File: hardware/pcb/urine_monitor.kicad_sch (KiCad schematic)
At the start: 27 parts, among them J1 LoadCell, J2 EInk_FPC, J3 USB-C_Power, Q1 SI2301, Q2 2N7002, SW1 USER_BTN, U1 RAK3172, U2 HX711, U3 TPS61220, U4 MIC5504-3.3

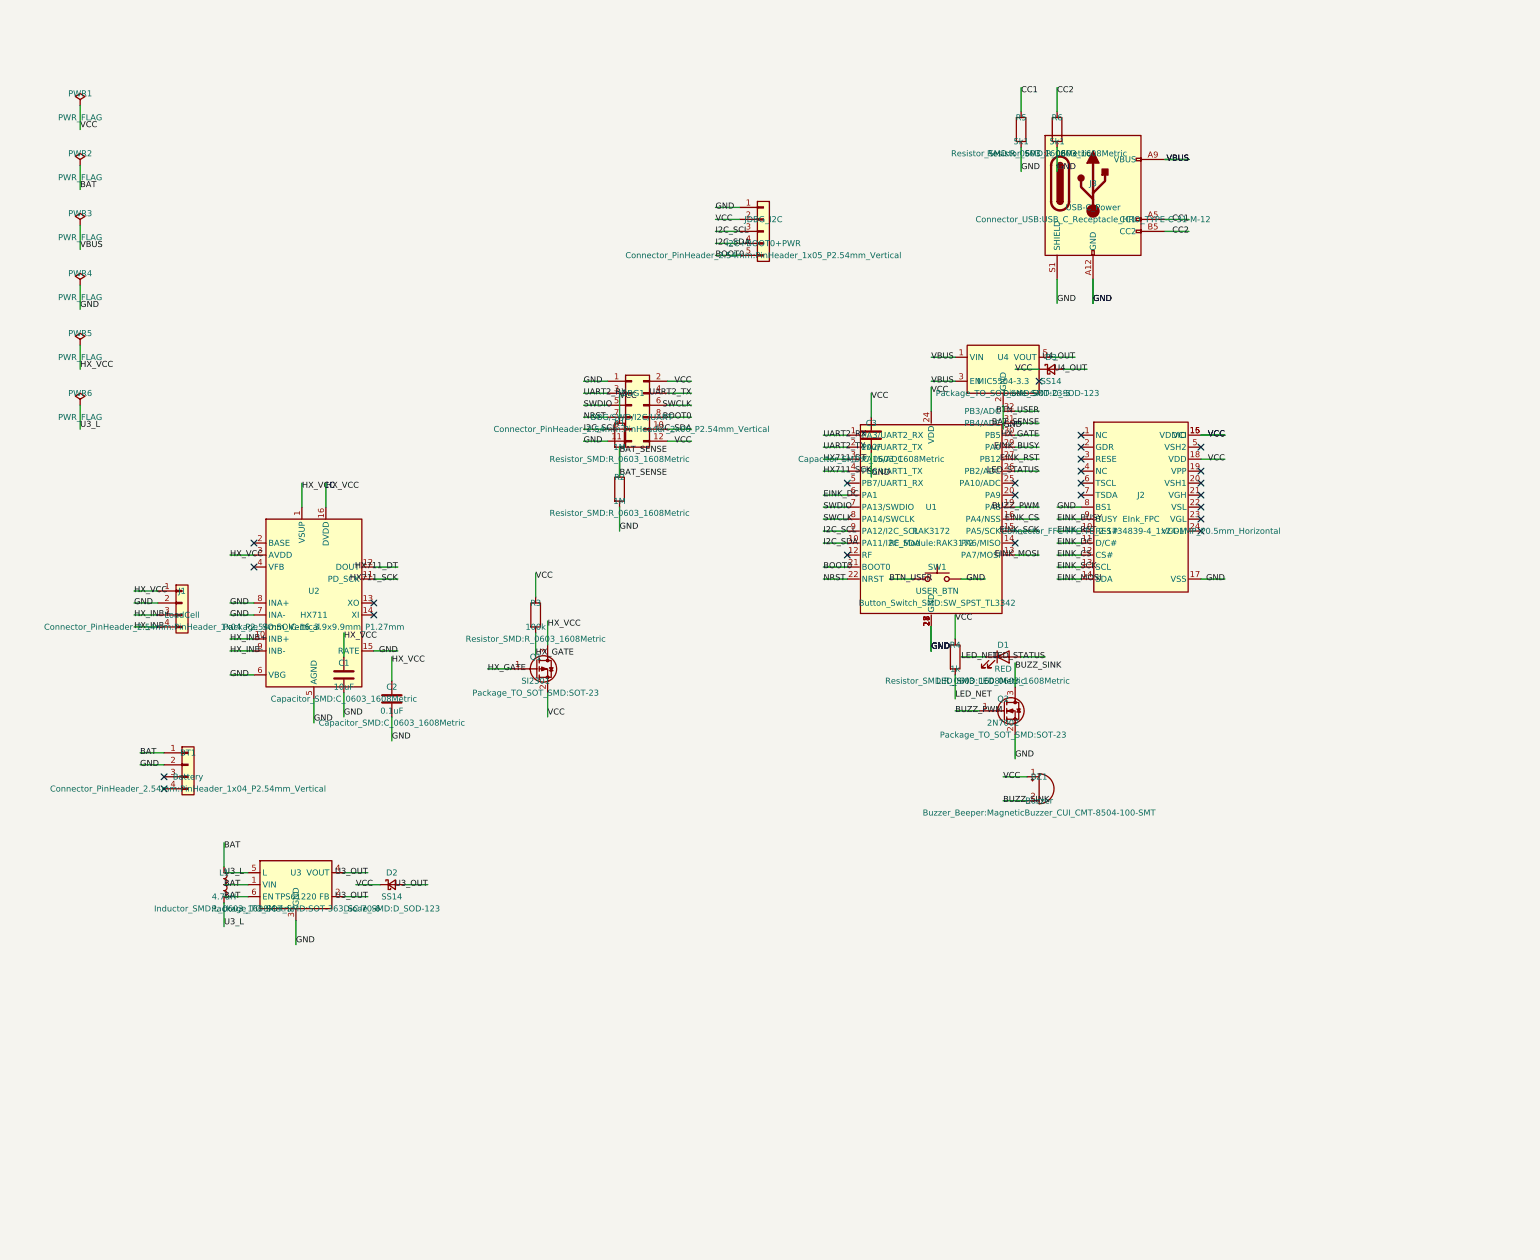
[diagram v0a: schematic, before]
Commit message: init
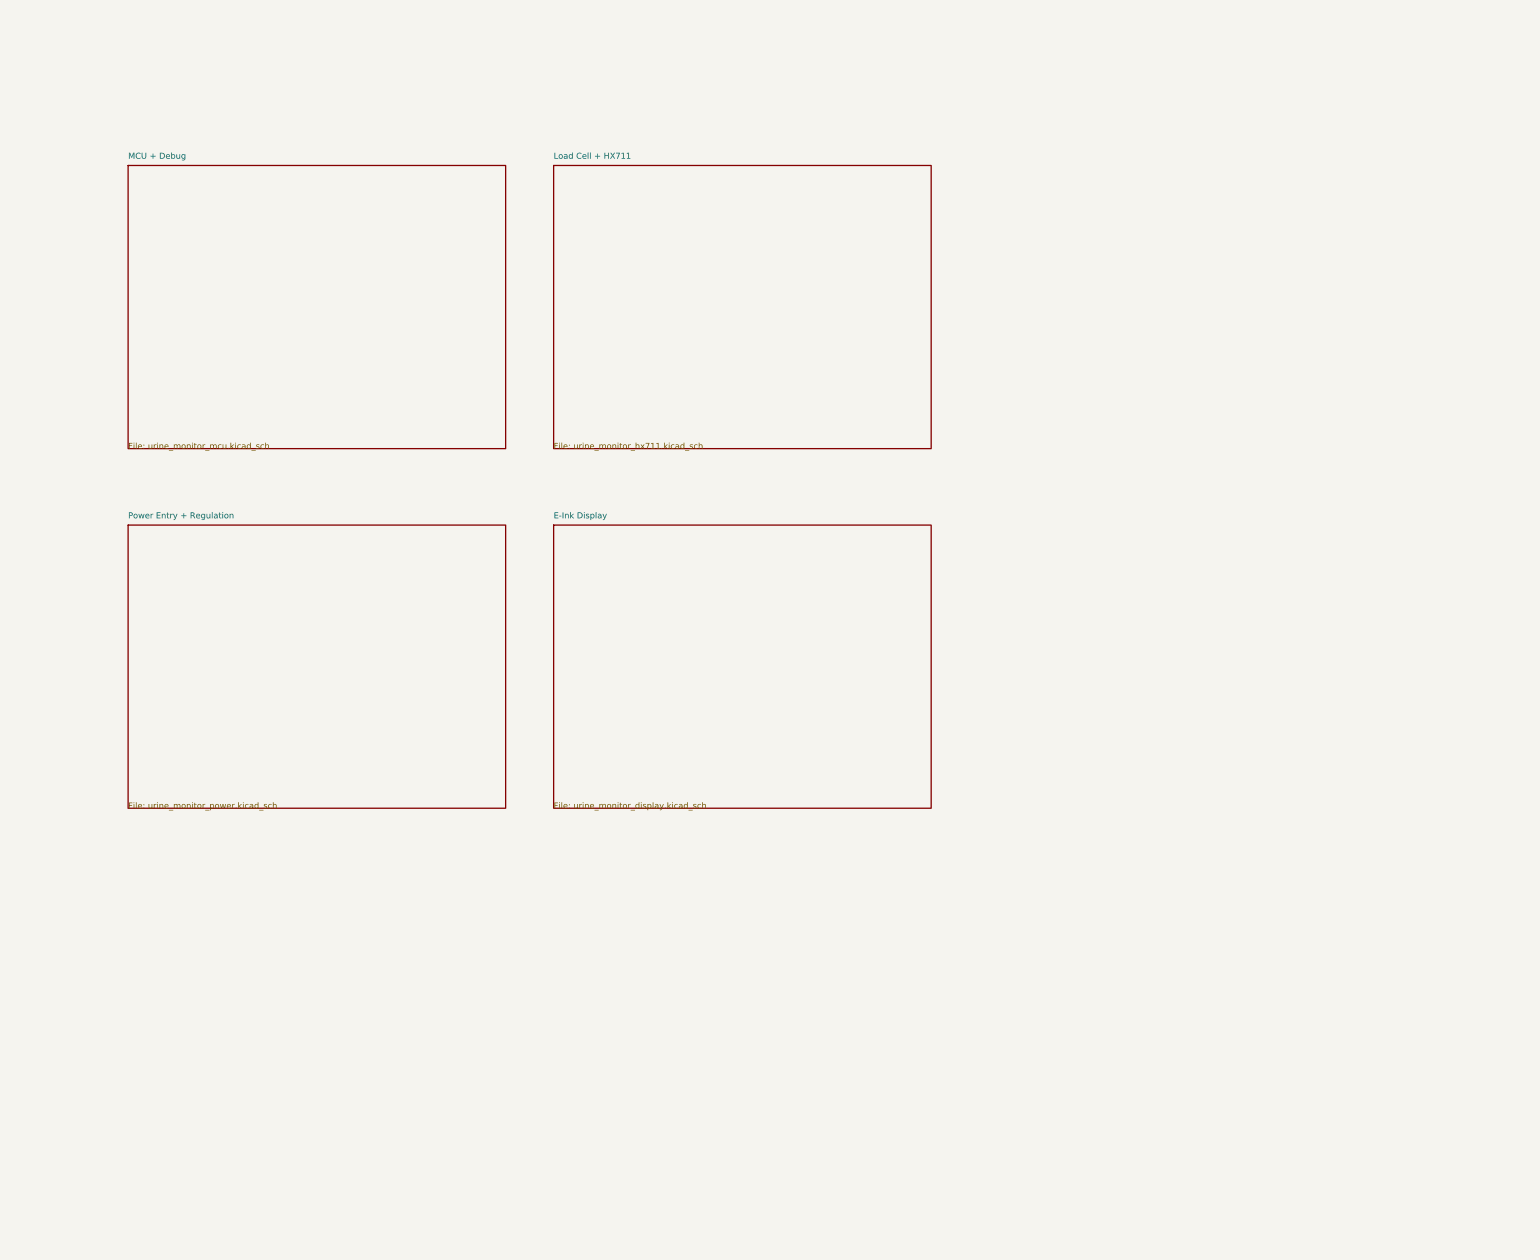
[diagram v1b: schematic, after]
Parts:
- removed BT1: Battery, Connector_PinHeader_2.54mm:PinHeader_1x04_P2.54mm_Vertical, symbol Connector_Generic:Conn_01x04
- removed BZ1: Buzzer, Buzzer_Beeper:MagneticBuzzer_CUI_CMT-8504-100-SMT, symbol Device:Buzzer
- removed C1, C3: 10uF, Capacitor_SMD:C_0603_1608Metric, symbol Device:C
- removed C2: 0.1uF, Capacitor_SMD:C_0603_1608Metric, symbol Device:C
- removed D1: RED, LED_SMD:LED_0603_1608Metric, symbol Device:LED
- removed D2, D3: SS14, Diode_SMD:D_SOD-123, symbol Device:D_Schottky_Small
- removed J1: LoadCell, Connector_PinHeader_2.54mm:PinHeader_1x04_P2.54mm_Vertical, symbol Connector_Generic:Conn_01x04
- removed J2: EInk_FPC, Connector_FFC-FPC:TE_2-1734839-4_1x24-1MP_P0.5mm_Horizontal, symbol Project_Lib:GDEY0213B74
- removed J3: USB-C_Power, Connector_USB:USB_C_Receptacle_HRO_TYPE-C-31-M-12, symbol Connector:USB_C_Receptacle_PowerOnly_6P
- removed JDBG1: DBG/SWD/I2C/UART, Connector_PinHeader_2.54mm:PinHeader_2x06_P2.54mm_Vertical, symbol Connector_Generic:Conn_02x06_Odd_Even
- removed JDBG_I2C: I2C+BOOT0+PWR, Connector_PinHeader_2.54mm:PinHeader_1x05_P2.54mm_Vertical, symbol Connector_Generic:Conn_01x05
- removed L1: 4.7uH, Inductor_SMD:L_0603_1608Metric, symbol Device:L
- removed Q1: SI2301, Package_TO_SOT_SMD:SOT-23, symbol Transistor_FET:Q_PMOS_GSD
- removed Q2: 2N7002, Package_TO_SOT_SMD:SOT-23, symbol Transistor_FET:Q_NMOS_GSD
- removed R1, R2: 1M, Resistor_SMD:R_0603_1608Metric, symbol Device:R
- removed R3: 100k, Resistor_SMD:R_0603_1608Metric, symbol Device:R
- removed R4: 1k, Resistor_SMD:R_0603_1608Metric, symbol Device:R
- removed R5, R6: 5k1, Resistor_SMD:R_0603_1608Metric, symbol Device:R
- removed SW1: USER_BTN, Button_Switch_SMD:SW_SPST_TL3342, symbol Switch:SW_Push
- removed U1: RAK3172, RF_Module:RAK3172, symbol Project_Lib:RAK3172
- removed U2: HX711, Package_SO:SOIC-16_3.9x9.9mm_P1.27mm, symbol Analog_ADC:HX711
- removed U3: TPS61220, Package_TO_SOT_SMD:SOT-363_SC-70-6, symbol Regulator_Switching:TPS61220DCK
- removed U4: MIC5504-3.3, Package_TO_SOT_SMD:SOT-23-5, symbol Regulator_Linear:MIC5504-3.3YM5
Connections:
- no-connect marks 25 -> 0
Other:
- added sheet E-Ink Display (urine_monitor_display.kicad_sch)
- added sheet Load Cell + HX711 (urine_monitor_hx711.kicad_sch)
- added sheet MCU + Debug (urine_monitor_mcu.kicad_sch)
- added sheet Power Entry + Regulation (urine_monitor_power.kicad_sch)
- title: (none) -> Urine Monitor

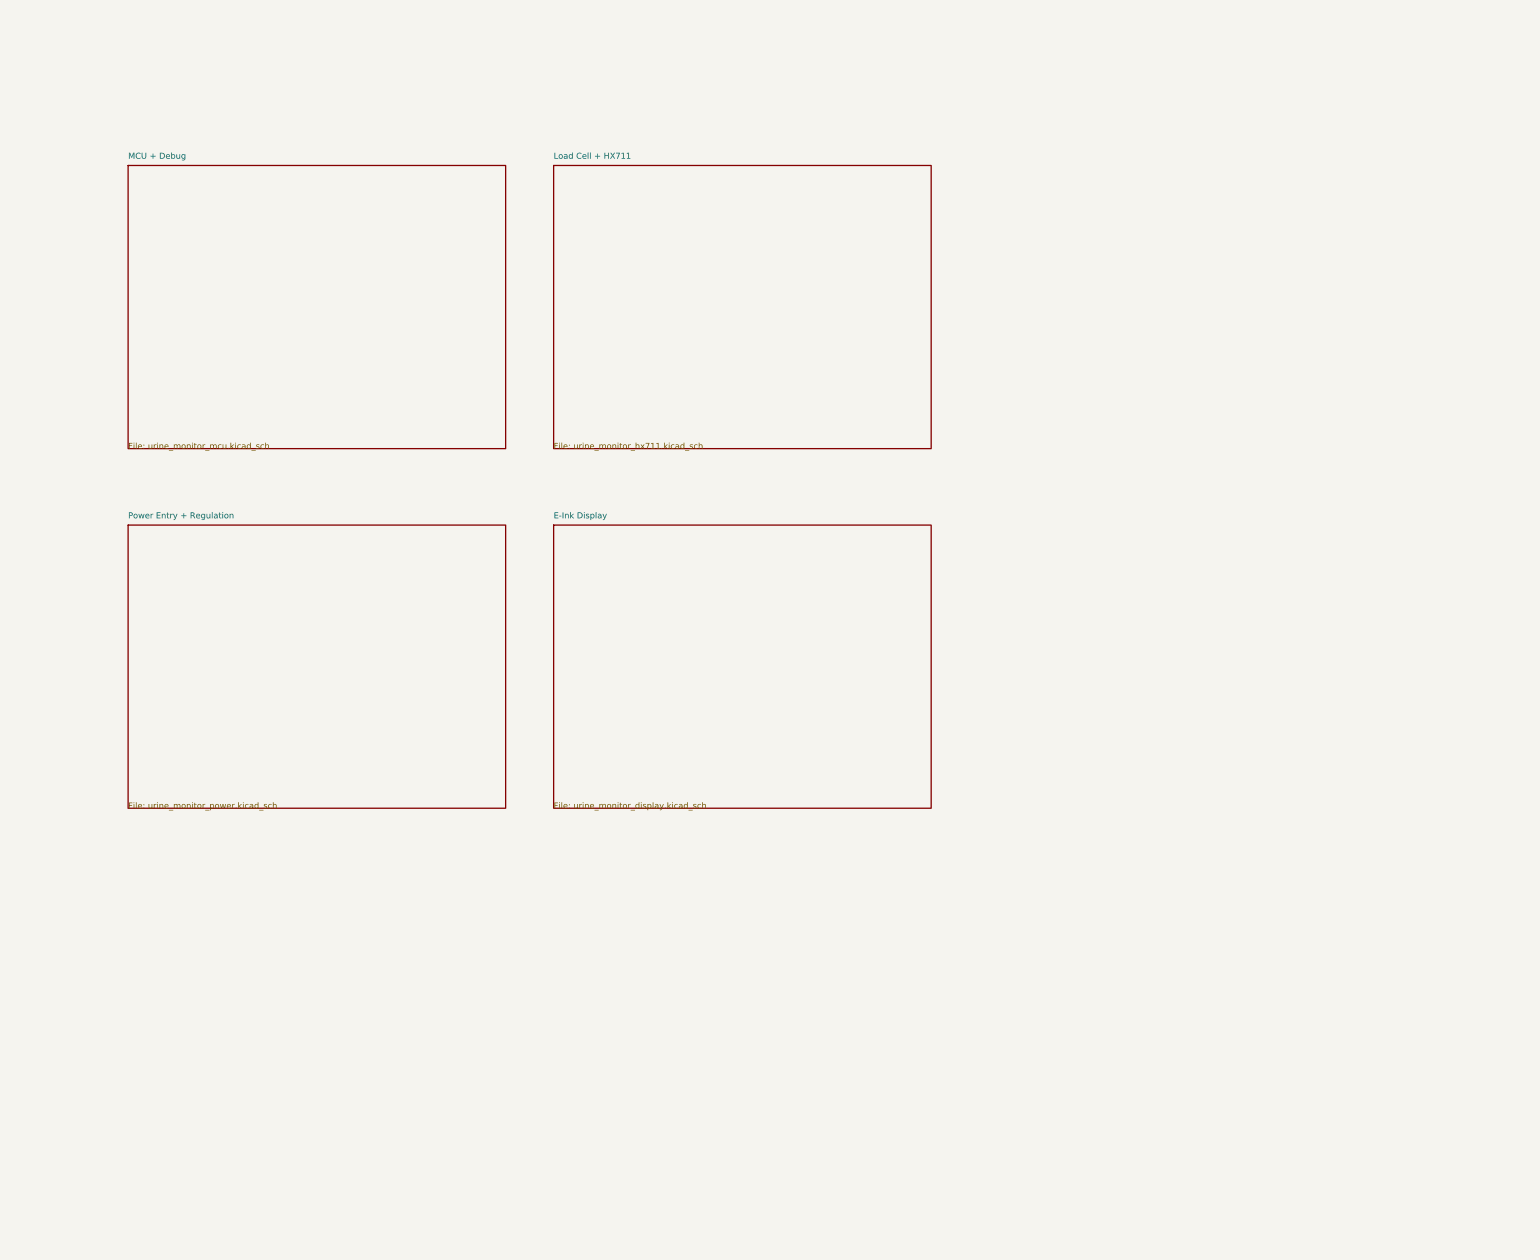
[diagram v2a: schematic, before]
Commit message: init
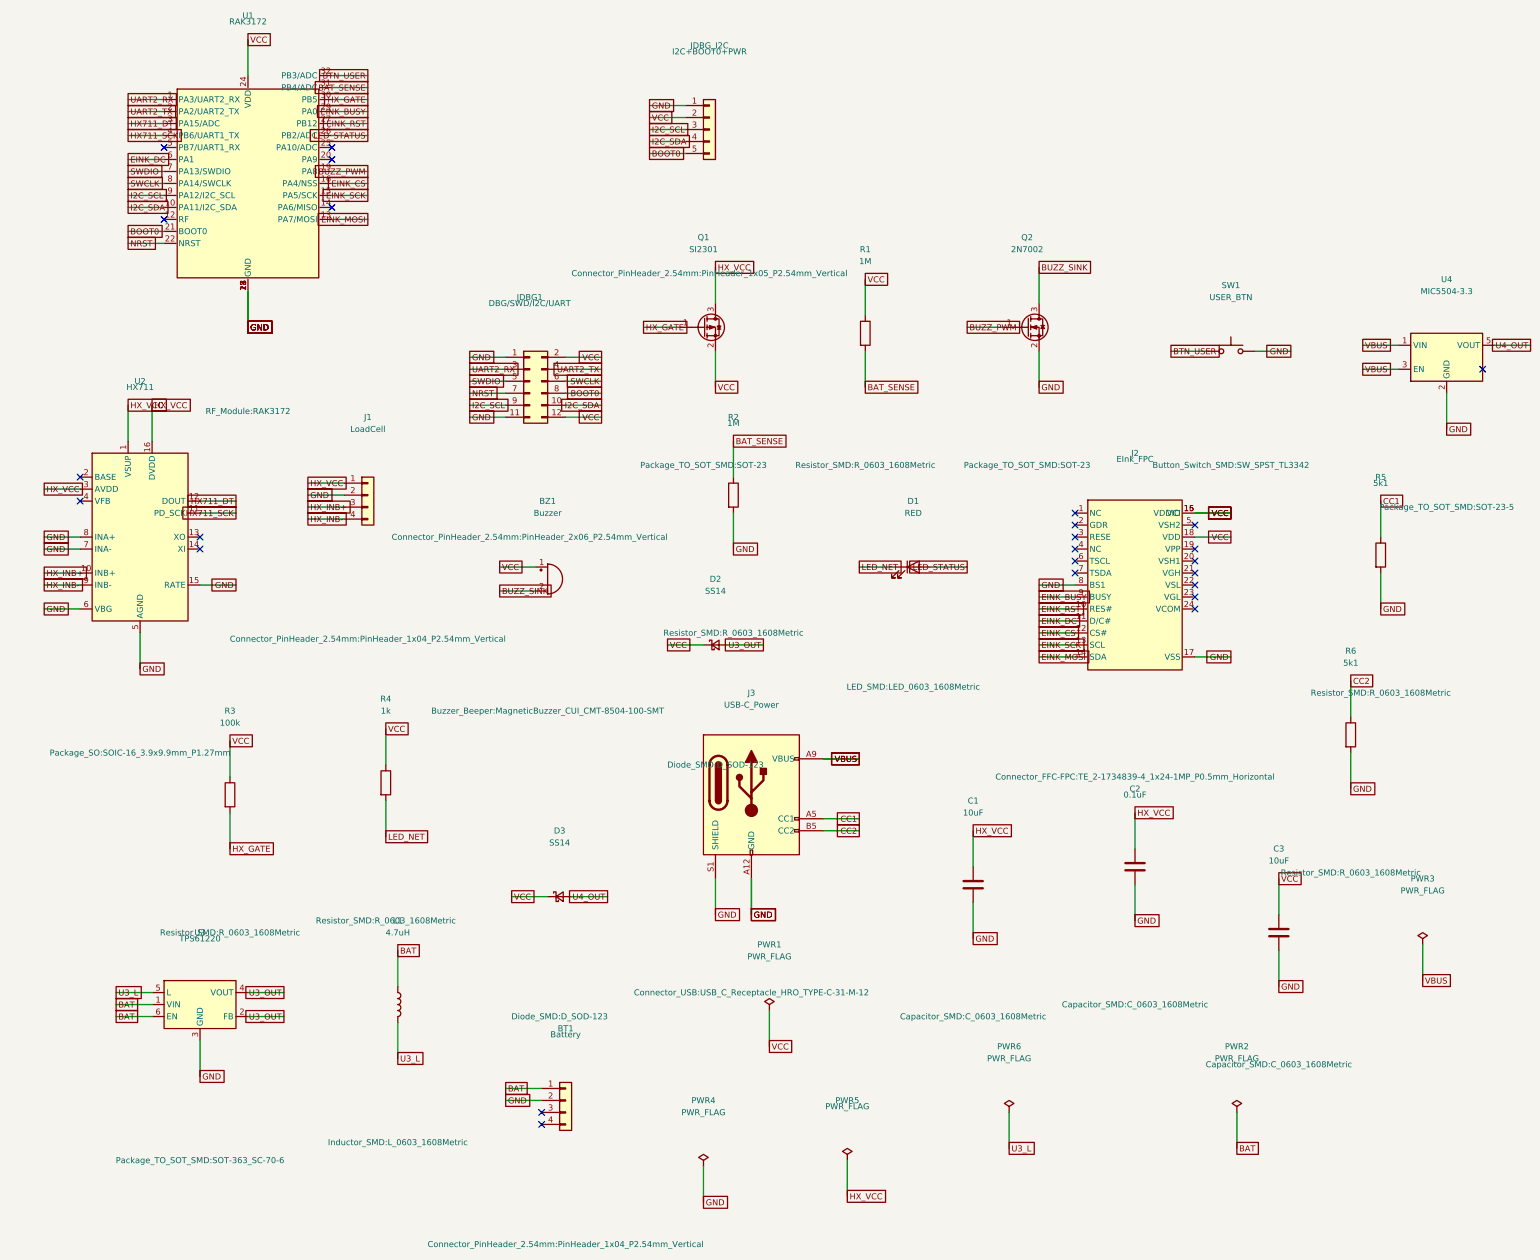
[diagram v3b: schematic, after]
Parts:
- added BT1: Battery, Connector_PinHeader_2.54mm:PinHeader_1x04_P2.54mm_Vertical, symbol Connector_Generic:Conn_01x04
- added BZ1: Buzzer, Buzzer_Beeper:MagneticBuzzer_CUI_CMT-8504-100-SMT, symbol Device:Buzzer
- added C1, C3: 10uF, Capacitor_SMD:C_0603_1608Metric, symbol Device:C
- added C2: 0.1uF, Capacitor_SMD:C_0603_1608Metric, symbol Device:C
- added D1: RED, LED_SMD:LED_0603_1608Metric, symbol Device:LED
- added D2, D3: SS14, Diode_SMD:D_SOD-123, symbol Device:D_Schottky_Small
- added J1: LoadCell, Connector_PinHeader_2.54mm:PinHeader_1x04_P2.54mm_Vertical, symbol Connector_Generic:Conn_01x04
- added J2: EInk_FPC, Connector_FFC-FPC:TE_2-1734839-4_1x24-1MP_P0.5mm_Horizontal, symbol Project_Lib:GDEY0213B74
- added J3: USB-C_Power, Connector_USB:USB_C_Receptacle_HRO_TYPE-C-31-M-12, symbol Connector:USB_C_Receptacle_PowerOnly_6P
- added JDBG1: DBG/SWD/I2C/UART, Connector_PinHeader_2.54mm:PinHeader_2x06_P2.54mm_Vertical, symbol Connector_Generic:Conn_02x06_Odd_Even
- added JDBG_I2C: I2C+BOOT0+PWR, Connector_PinHeader_2.54mm:PinHeader_1x05_P2.54mm_Vertical, symbol Connector_Generic:Conn_01x05
- added L1: 4.7uH, Inductor_SMD:L_0603_1608Metric, symbol Device:L
- added Q1: SI2301, Package_TO_SOT_SMD:SOT-23, symbol Transistor_FET:Q_PMOS_GSD
- added Q2: 2N7002, Package_TO_SOT_SMD:SOT-23, symbol Transistor_FET:Q_NMOS_GSD
- added R1, R2: 1M, Resistor_SMD:R_0603_1608Metric, symbol Device:R
- added R3: 100k, Resistor_SMD:R_0603_1608Metric, symbol Device:R
- added R4: 1k, Resistor_SMD:R_0603_1608Metric, symbol Device:R
- added R5, R6: 5k1, Resistor_SMD:R_0603_1608Metric, symbol Device:R
- added SW1: USER_BTN, Button_Switch_SMD:SW_SPST_TL3342, symbol Switch:SW_Push
- added U1: RAK3172, RF_Module:RAK3172, symbol Project_Lib:RAK3172
- added U2: HX711, Package_SO:SOIC-16_3.9x9.9mm_P1.27mm, symbol Analog_ADC:HX711
- added U3: TPS61220, Package_TO_SOT_SMD:SOT-363_SC-70-6, symbol Regulator_Switching:TPS61220DCK
- added U4: MIC5504-3.3, Package_TO_SOT_SMD:SOT-23-5, symbol Regulator_Linear:MIC5504-3.3YM5
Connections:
- new net BAT: BT1.1 (Pin_1), L1.1, U3.1 (VIN), U3.6 (EN)
- new net BAT_SENSE: R1.2, R2.1, U1.31 (PB4/ADC)
- new net BOOT0: JDBG1.8 (Pin_8), JDBG_I2C.5 (Pin_5), U1.21 (BOOT0)
- new net BTN_USER: SW1.1, U1.32 (PB3/ADC)
- new net BUZZ_PWM: Q2.1 (G), U1.19 (PA8)
- new net BUZZ_SINK: BZ1.2 (-), Q2.3 (D)
- new net CC1: J3.A5 (CC1), R5.1
- new net CC2: J3.B5 (CC2), R6.1
- new net EINK_BUSY: J2.9 (BUSY), U1.29 (PA0)
- new net EINK_CS: J2.12 (CS#), U1.16 (PA4/NSS)
- new net EINK_DC: J2.11 (D/C#), U1.6 (PA1)
- new net EINK_MOSI: J2.14 (SDA), U1.13 (PA7/MOSI)
- new net EINK_RST: J2.10 (RES#), U1.27 (PB12)
- new net EINK_SCK: J2.13 (SCL), U1.15 (PA5/SCK)
- new net GND: BT1.2 (Pin_2), C1.2, C2.2, C3.2, J1.2 (Pin_2), J2.17 (VSS), J2.8 (BS1), J3.A12 (GND), J3.B12 (GND), J3.S1 (SHIELD), JDBG1.1 (Pin_1), JDBG1.11 (Pin_11), JDBG_I2C.1 (Pin_1), Q2.2 (S), R2.2, R5.2, R6.2, SW1.2, U1.11 (GND), U1.17 (GND), U1.18 (GND), U1.23 (GND), U1.28 (GND), U2.15 (RATE), U2.5 (AGND), U2.6 (VBG), U2.7 (INA-), U2.8 (INA+), U3.3 (GND), U4.2 (GND)
- new net HX711_DT: U1.3 (PA15/ADC), U2.12 (DOUT)
- new net HX711_SCK: U1.4 (PB6/UART1_TX), U2.11 (PD_SCK)
- new net HX_GATE: Q1.1 (G), R3.2, U1.30 (PB5)
- new net HX_INB+: J1.3 (Pin_3), U2.10 (INB+)
- new net HX_INB-: J1.4 (Pin_4), U2.9 (INB-)
- new net HX_VCC: C1.1, C2.1, J1.1 (Pin_1), Q1.3 (D), U2.1 (VSUP), U2.16 (DVDD), U2.3 (AVDD)
- new net I2C_SCL: JDBG1.9 (Pin_9), JDBG_I2C.3 (Pin_3), U1.9 (PA12/I2C_SCL)
- new net I2C_SDA: JDBG1.10 (Pin_10), JDBG_I2C.4 (Pin_4), U1.10 (PA11/I2C_SDA)
- new net LED_NET: D1.1 (K), R4.2
- new net LED_STATUS: D1.2 (A), U1.26 (PB2/ADC)
- new net NRST: JDBG1.7 (Pin_7), U1.22 (NRST)
- new net SWCLK: JDBG1.6 (Pin_6), U1.8 (PA14/SWCLK)
- new net SWDIO: JDBG1.5 (Pin_5), U1.7 (PA13/SWDIO)
- new net U3_L: L1.2, U3.5 (L)
- new net U3_OUT: D2.2 (A), U3.2 (FB), U3.4 (VOUT)
- new net U4_OUT: D3.2 (A), U4.5 (VOUT)
- new net UART2_RX: JDBG1.3 (Pin_3), U1.1 (PA3/UART2_RX)
- new net UART2_TX: JDBG1.4 (Pin_4), U1.2 (PA2/UART2_TX)
- new net VBUS: J3.A9 (VBUS), J3.B9 (VBUS), U4.1 (VIN), U4.3 (EN)
- new net VCC: BZ1.1 (+), C3.1, D2.1 (K), D3.1 (K), J2.15 (VDDIO), J2.16 (VCI), J2.18 (VDD), JDBG1.12 (Pin_12), JDBG1.2 (Pin_2), JDBG_I2C.2 (Pin_2), Q1.2 (S), R1.1, R3.1, R4.1, U1.24 (VDD)
- no-connect marks 0 -> 25
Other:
- removed sheet E-Ink Display
- removed sheet Load Cell + HX711
- removed sheet MCU + Debug
- removed sheet Power Entry + Regulation
